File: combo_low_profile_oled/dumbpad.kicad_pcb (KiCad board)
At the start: 2 copper layers, 97 x 78.5 mm, 45 parts, among them J1 Conn_01x04_Female

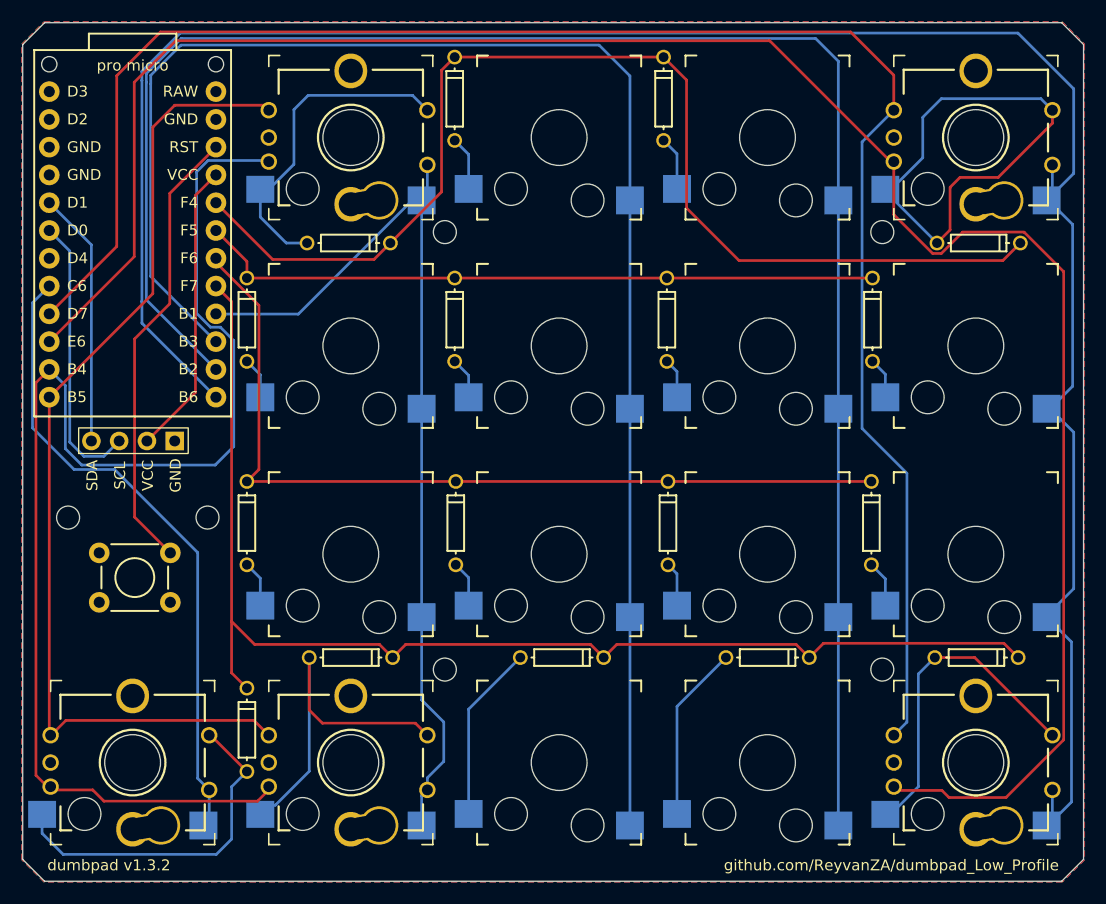
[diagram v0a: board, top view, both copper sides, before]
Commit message: Added images for completed keypad v1.3.1
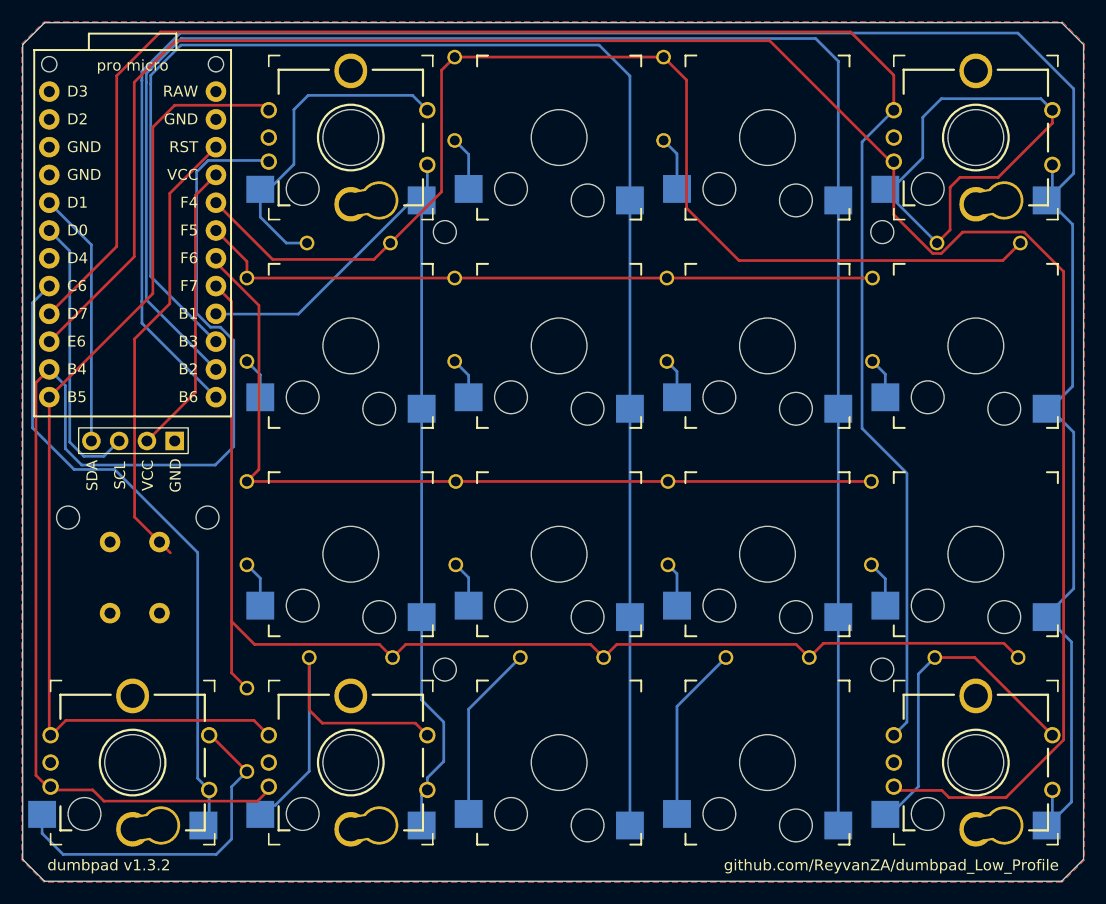
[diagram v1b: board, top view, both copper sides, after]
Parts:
- D1, D10, D11, D12, D13, D14, D15, D16, D2, D20, D3, D4, D5, D6, D7, D8, D9, S17: moved to B.Cu
- turned S17 to -90 degrees
